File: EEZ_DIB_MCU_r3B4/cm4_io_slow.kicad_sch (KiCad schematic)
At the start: 1 part

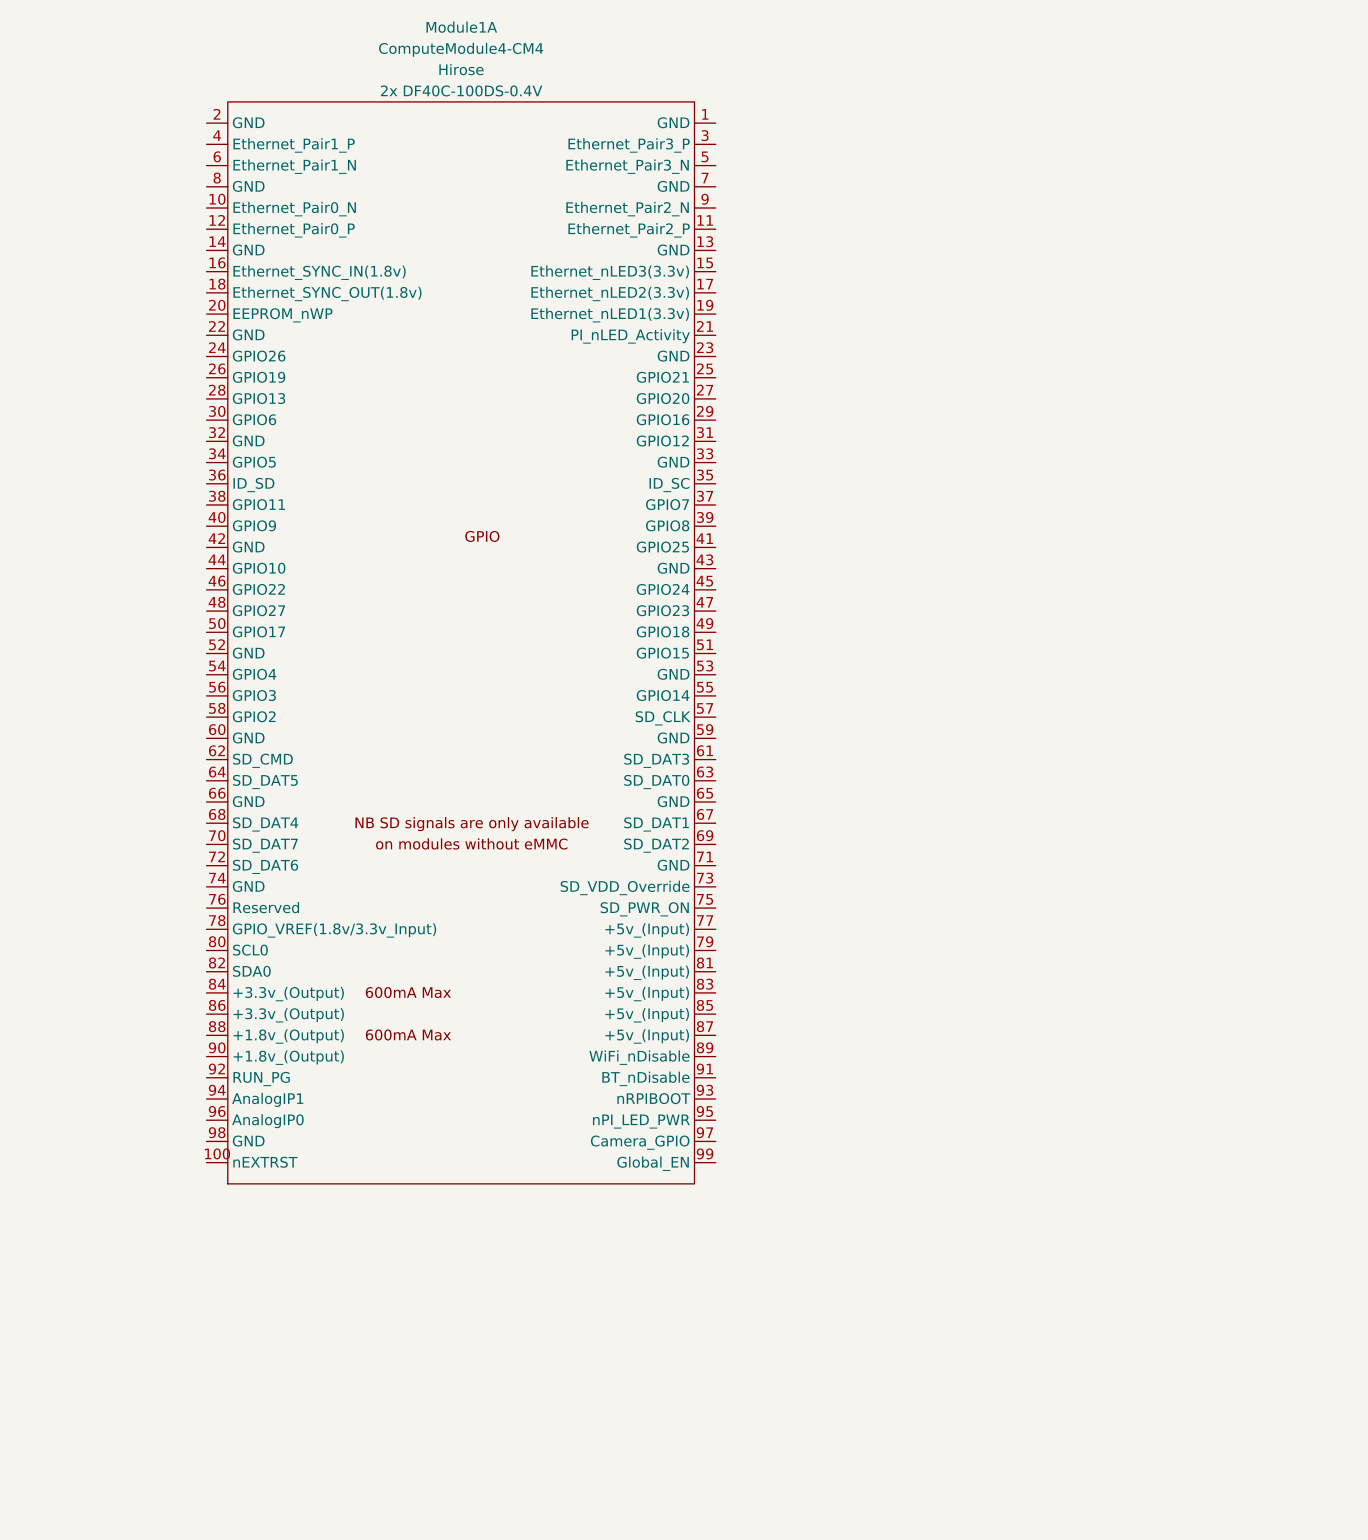
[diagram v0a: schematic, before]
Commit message: Splitting SoM and MCU board
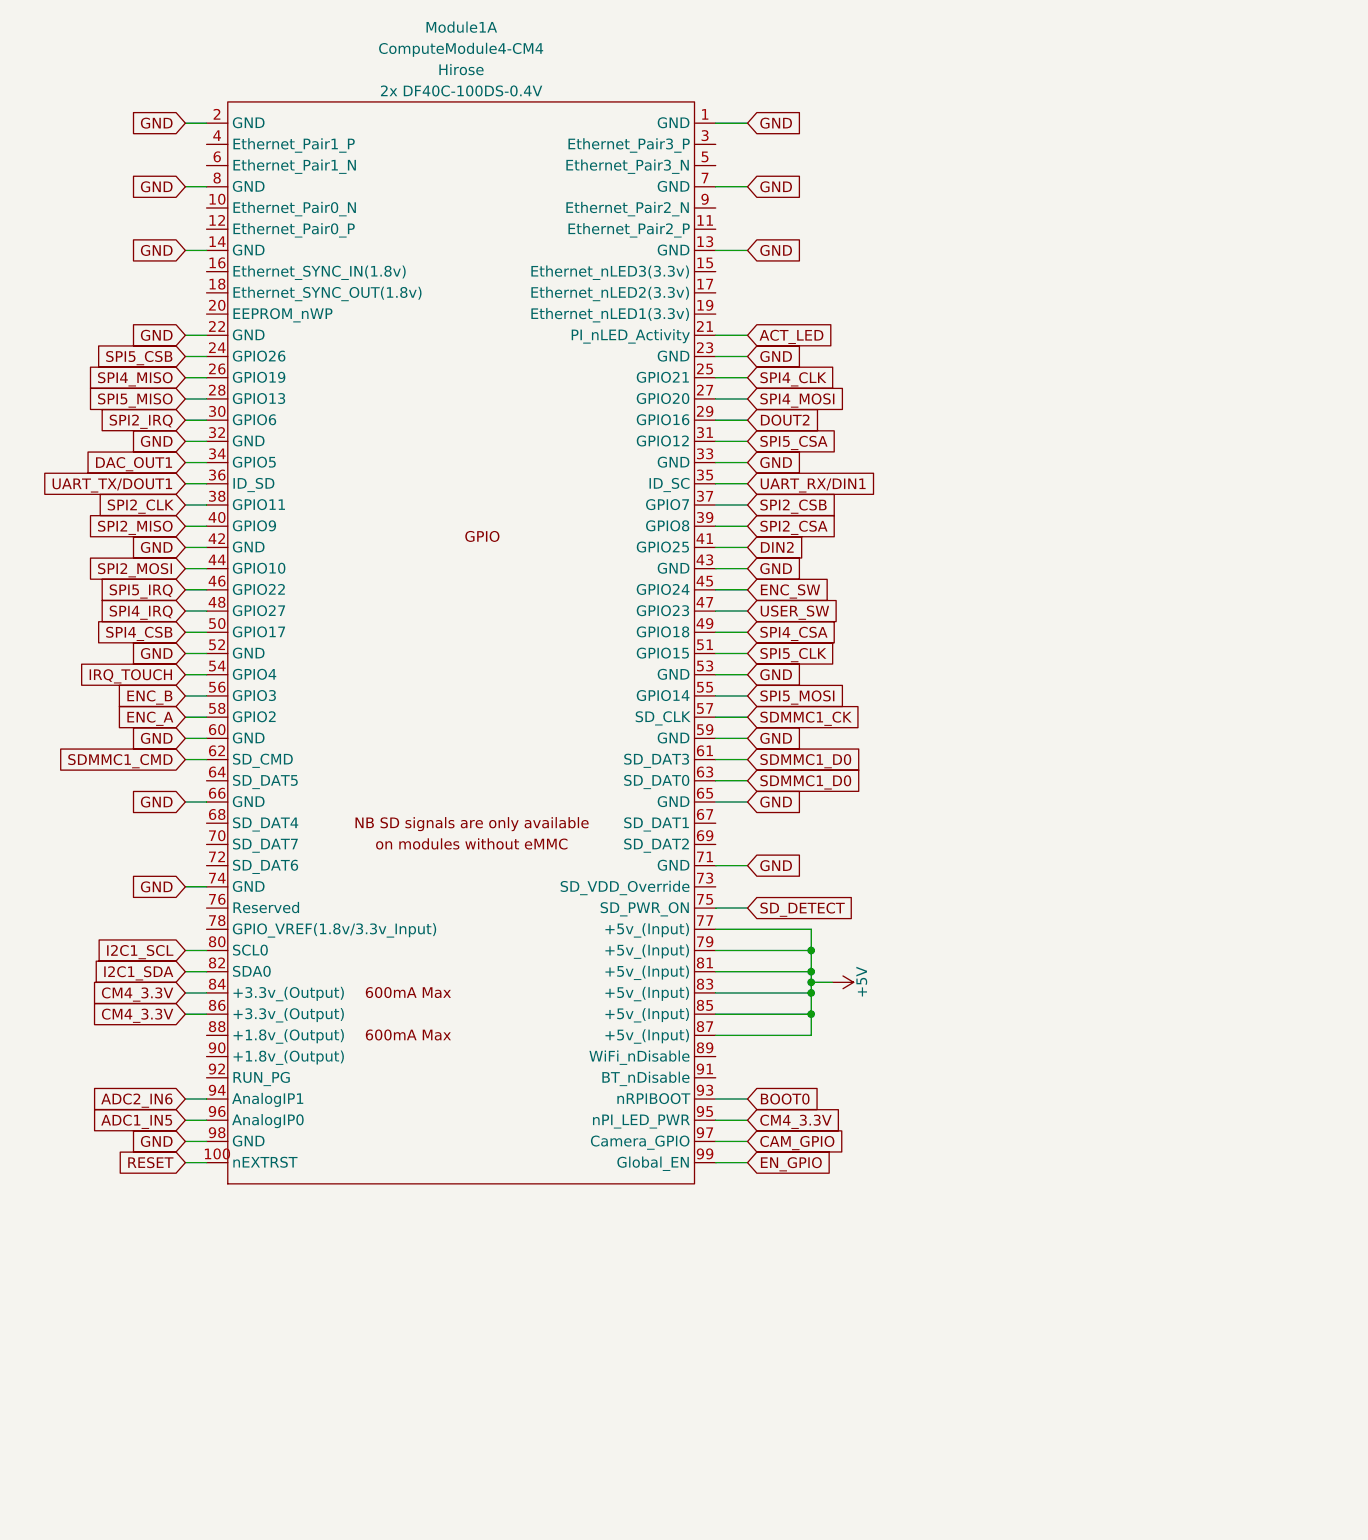
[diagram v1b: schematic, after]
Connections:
- net GND: now reaches Module1.1 (GND)
- net GND: now also Module1.13 (GND), Module1.14 (GND), Module1.2 (GND), Module1.22 (GND), Module1.23 (GND), Module1.32 (GND), Module1.33 (GND), Module1.42 (GND), Module1.43 (GND), Module1.52 (GND), Module1.53 (GND), Module1.59 (GND), Module1.60 (GND), Module1.65 (GND), Module1.66 (GND), Module1.7 (GND), Module1.71 (GND), Module1.74 (GND), Module1.8 (GND), Module1.98 (GND)
- net RESET: now reaches Module1.100 (nEXTRST)
- net ACT_LED: now reaches Module1.21 (PI_nLED_Activity)
- net SPI5_CSB: now reaches Module1.24 (GPIO26)
- net SPI4_CLK: now reaches Module1.25 (GPIO21)
- net SPI4_MISO: now reaches Module1.26 (GPIO19)
- net SPI4_MOSI: now reaches Module1.27 (GPIO20)
- net SPI5_MISO: now reaches Module1.28 (GPIO13)
- net DOUT2: now reaches Module1.29 (GPIO16)
- net SPI2_IRQ: now reaches Module1.30 (GPIO6)
- net SPI5_CSA: now reaches Module1.31 (GPIO12)
- net DAC_OUT1: now reaches Module1.34 (GPIO5)
- net UART_RX/DIN1: now reaches Module1.35 (ID_SC)
- net UART_TX/DOUT1: now reaches Module1.36 (ID_SD)
- net SPI2_CSB: now reaches Module1.37 (GPIO7)
- net SPI2_CLK: now reaches Module1.38 (GPIO11)
- net SPI2_CSA: now reaches Module1.39 (GPIO8)
- net SPI2_MISO: now reaches Module1.40 (GPIO9)
- net DIN2: now reaches Module1.41 (GPIO25)
- net SPI2_MOSI: now reaches Module1.44 (GPIO10)
- net ENC_SW: now reaches Module1.45 (GPIO24)
- net SPI5_IRQ: now reaches Module1.46 (GPIO22)
- net USER_SW: now reaches Module1.47 (GPIO23)
- net SPI4_IRQ: now reaches Module1.48 (GPIO27)
- net SPI4_CSA: now reaches Module1.49 (GPIO18)
- net SPI4_CSB: now reaches Module1.50 (GPIO17)
- net SPI5_CLK: now reaches Module1.51 (GPIO15)
- net IRQ_TOUCH: now reaches Module1.54 (GPIO4)
- net SPI5_MOSI: now reaches Module1.55 (GPIO14)
- net ENC_B: now reaches Module1.56 (GPIO3)
- net SDMMC1_CK: now reaches Module1.57 (SD_CLK)
- net ENC_A: now reaches Module1.58 (GPIO2)
- net SDMMC1_D0: now reaches Module1.61 (SD_DAT3)
- net SDMMC1_D0: now also Module1.63 (SD_DAT0)
- net SDMMC1_CMD: now reaches Module1.62 (SD_CMD)
- net SD_DETECT: now reaches Module1.75 (SD_PWR_ON)
- net +5V: now reaches Module1.77 (+5v_(Input))
- net +5V: now also Module1.79 (+5v_(Input)), Module1.81 (+5v_(Input)), Module1.83 (+5v_(Input)), Module1.85 (+5v_(Input)), Module1.87 (+5v_(Input))
- net I2C1_SCL: now reaches Module1.80 (SCL0)
- net I2C1_SDA: now reaches Module1.82 (SDA0)
- net CM4_3.3V: now reaches Module1.84 (+3.3v_(Output))
- net CM4_3.3V: now also Module1.86 (+3.3v_(Output)), Module1.95 (nPI_LED_PWR)
- net BOOT0: now reaches Module1.93 (nRPIBOOT)
- net ADC2_IN6: now reaches Module1.94 (AnalogIP1)
- net ADC1_IN5: now reaches Module1.96 (AnalogIP0)
- net CAM_GPIO: now reaches Module1.97 (Camera_GPIO)
- net EN_GPIO: now reaches Module1.99 (Global_EN)

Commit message: Adding ICN6211
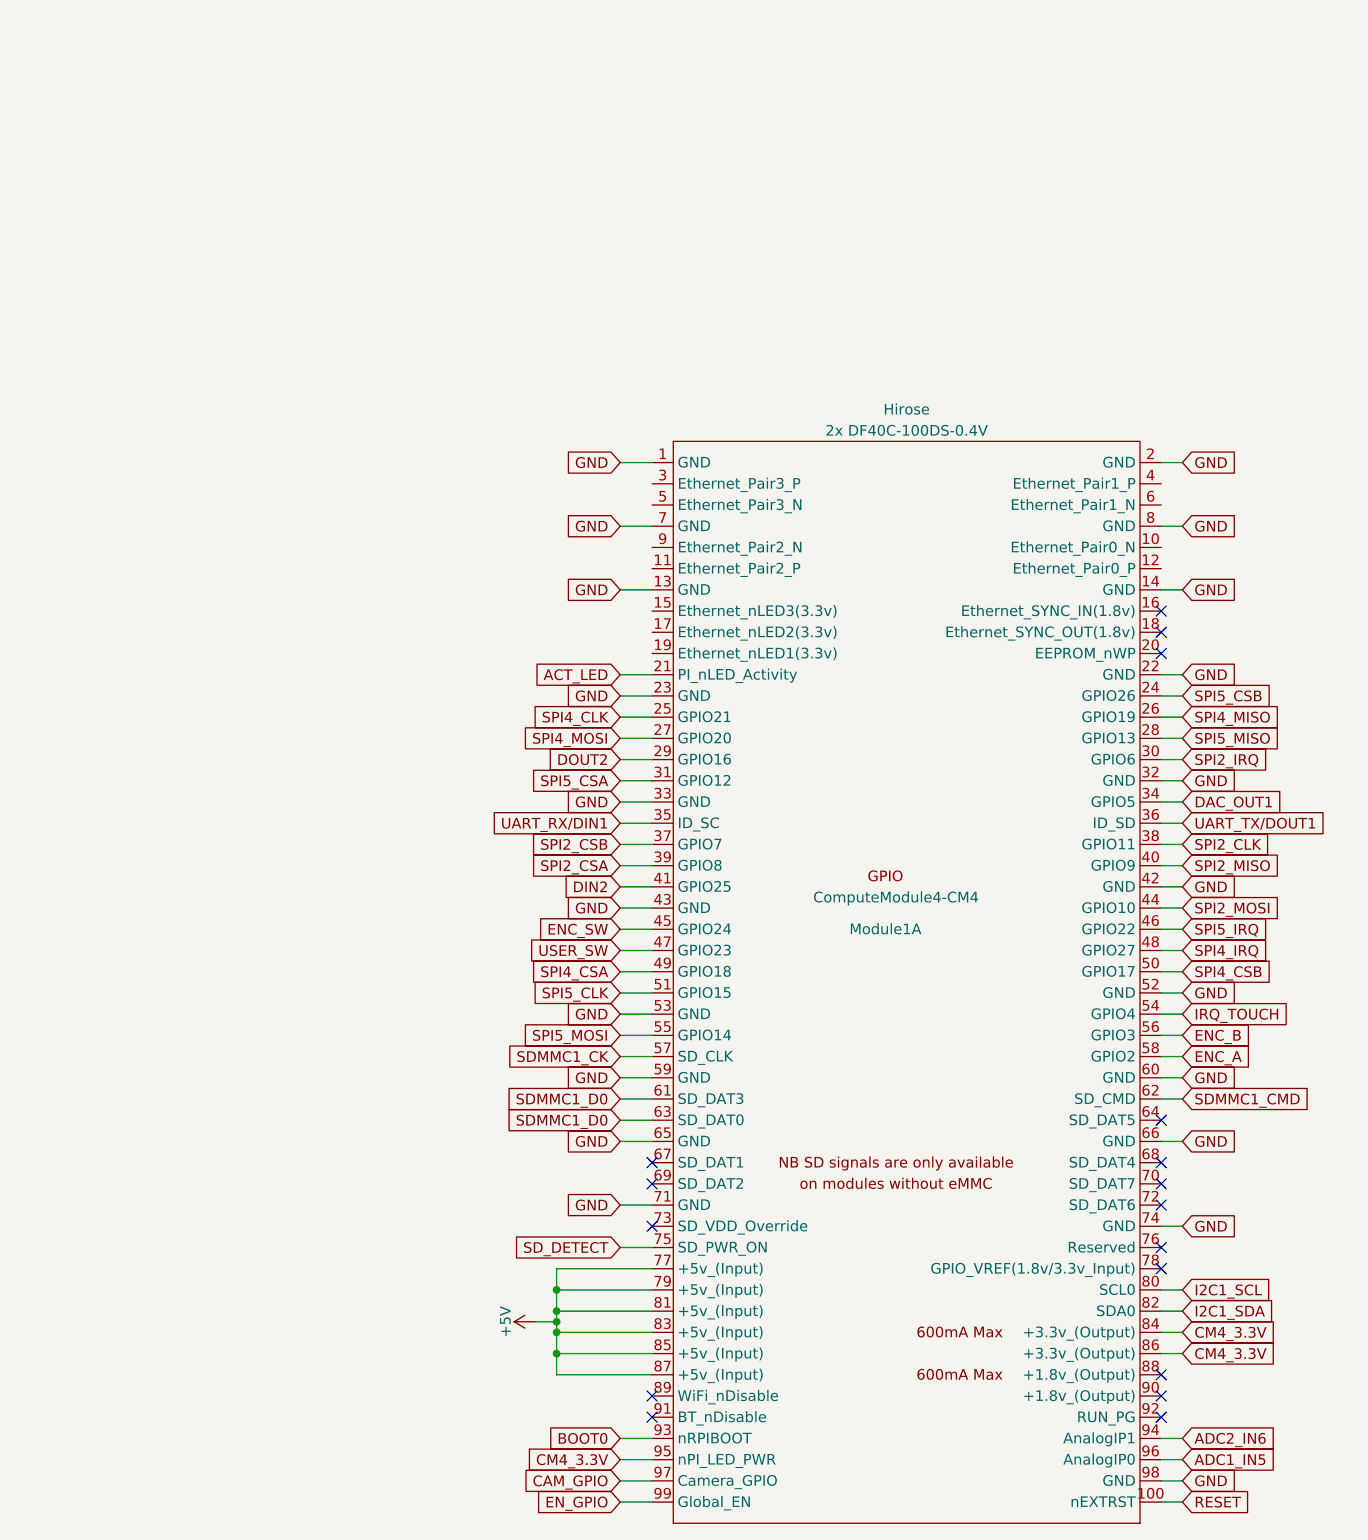
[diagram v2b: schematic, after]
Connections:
- no-connect marks 0 -> 17
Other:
- moved on the sheet: Module1A
